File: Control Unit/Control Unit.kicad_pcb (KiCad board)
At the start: 2 copper layers, 98.5 x 63.5 mm, 18 parts, among them J1 Conn_01x03_Pin, J2 LM2596S, J3 ST7789, J4 DHT20, J5 RTC, J6 RPM_IN, J7 Page flip, K1 Relay_SPDT, SW1 SW_DPST_x2, U1 ESP32-DEVKIT-V1, U2 PC817

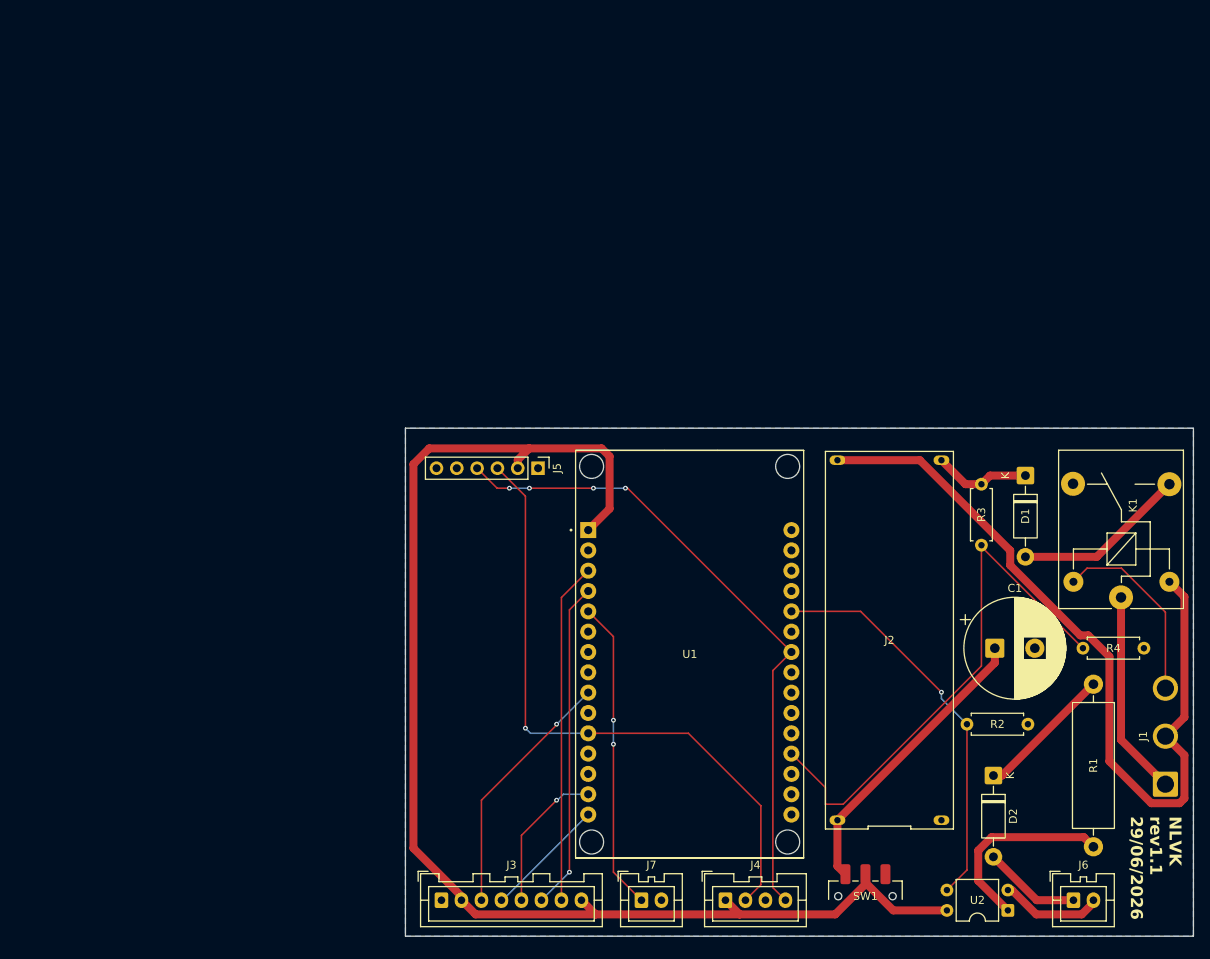
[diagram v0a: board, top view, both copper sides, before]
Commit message: rev1.1: polished user interface
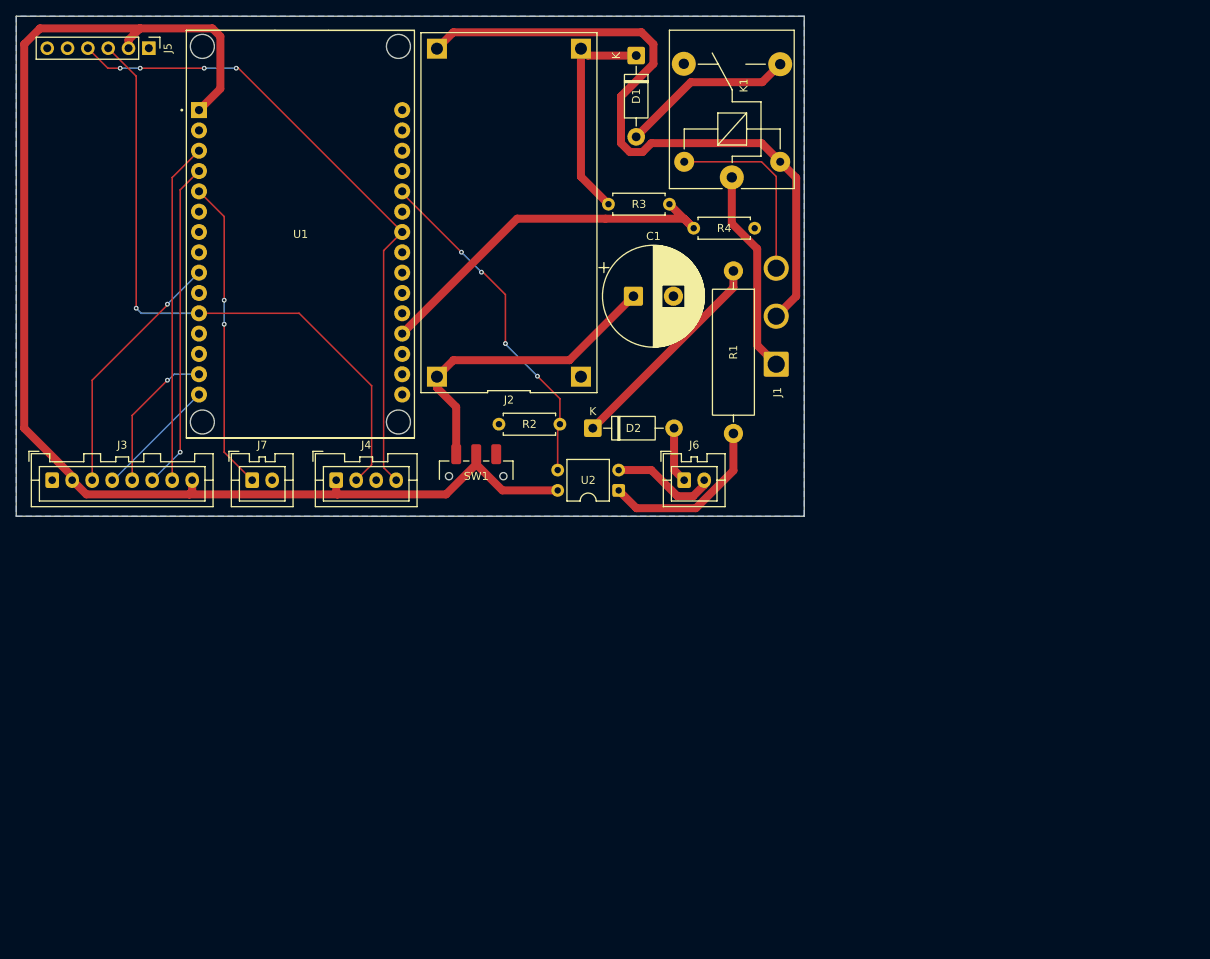
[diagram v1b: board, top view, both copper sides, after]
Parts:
- moved K1 71.6 mm to (142.3, 48.6)
- moved U1 71.6 mm to (88.4, 55.8)
- moved D1 71.6 mm to (130.3, 33.4)
- moved J1 71.6 mm to (147.8, 72.0)
- moved J3 71.6 mm to (57.3, 86.5)
- moved J4 71.6 mm to (92.8, 86.5)
- moved J5 71.6 mm to (69.4, 32.5)
- moved J6 71.6 mm to (136.3, 86.5)
- moved J7 71.6 mm to (82.3, 86.5)
- moved R4 71.6 mm to (145.2, 55.0)
- moved SW1 71.6 mm to (110.3, 86.0)
- moved U2 71.6 mm to (128.2, 87.8)
- moved J2 71.5 mm to (114.4, 53.1)
- moved R1 68.5 mm to (142.5, 60.3)
- moved D2 66.3 mm to (124.9, 80.0), turned to 0 degrees
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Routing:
- net Net-(U1-D34): track 68.0 -> 47.2 mm
- net /12V_PWR: track 12.2 -> 28.1 mm
- net /12V_GND: track 99.9 -> 85.5 mm
- net /RPM_PWR_RESISTOR: track 17.2 -> 26.9 mm
- net Net-(U1-D14): track 50.0 -> 43.2 mm, vias 1 -> 4
- net /RPM_PWR_DIODE: track 12.2 -> 7.02 mm
- net /RPM_PWR: track 24.6 -> 21.9 mm
- net /3.3V_PWR_SW: track 36.8 -> 39.4 mm
- net /3.3V_PWR: track 167.9 -> 165.5 mm
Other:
- board size 98.5 x 63.5 mm -> 98.5 x 62.5 mm
- board text added: "Motocycle Telemetry Sensor Made by: Nguyen Lam Vinh Khang rev1.1 30/06/2026"
- board text removed: "NLVK rev1.1 29/06/2026"
